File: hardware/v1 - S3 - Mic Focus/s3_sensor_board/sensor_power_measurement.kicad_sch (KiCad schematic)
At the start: 9 parts, among them J501 Conn_01x05, J502 Conn_01x05

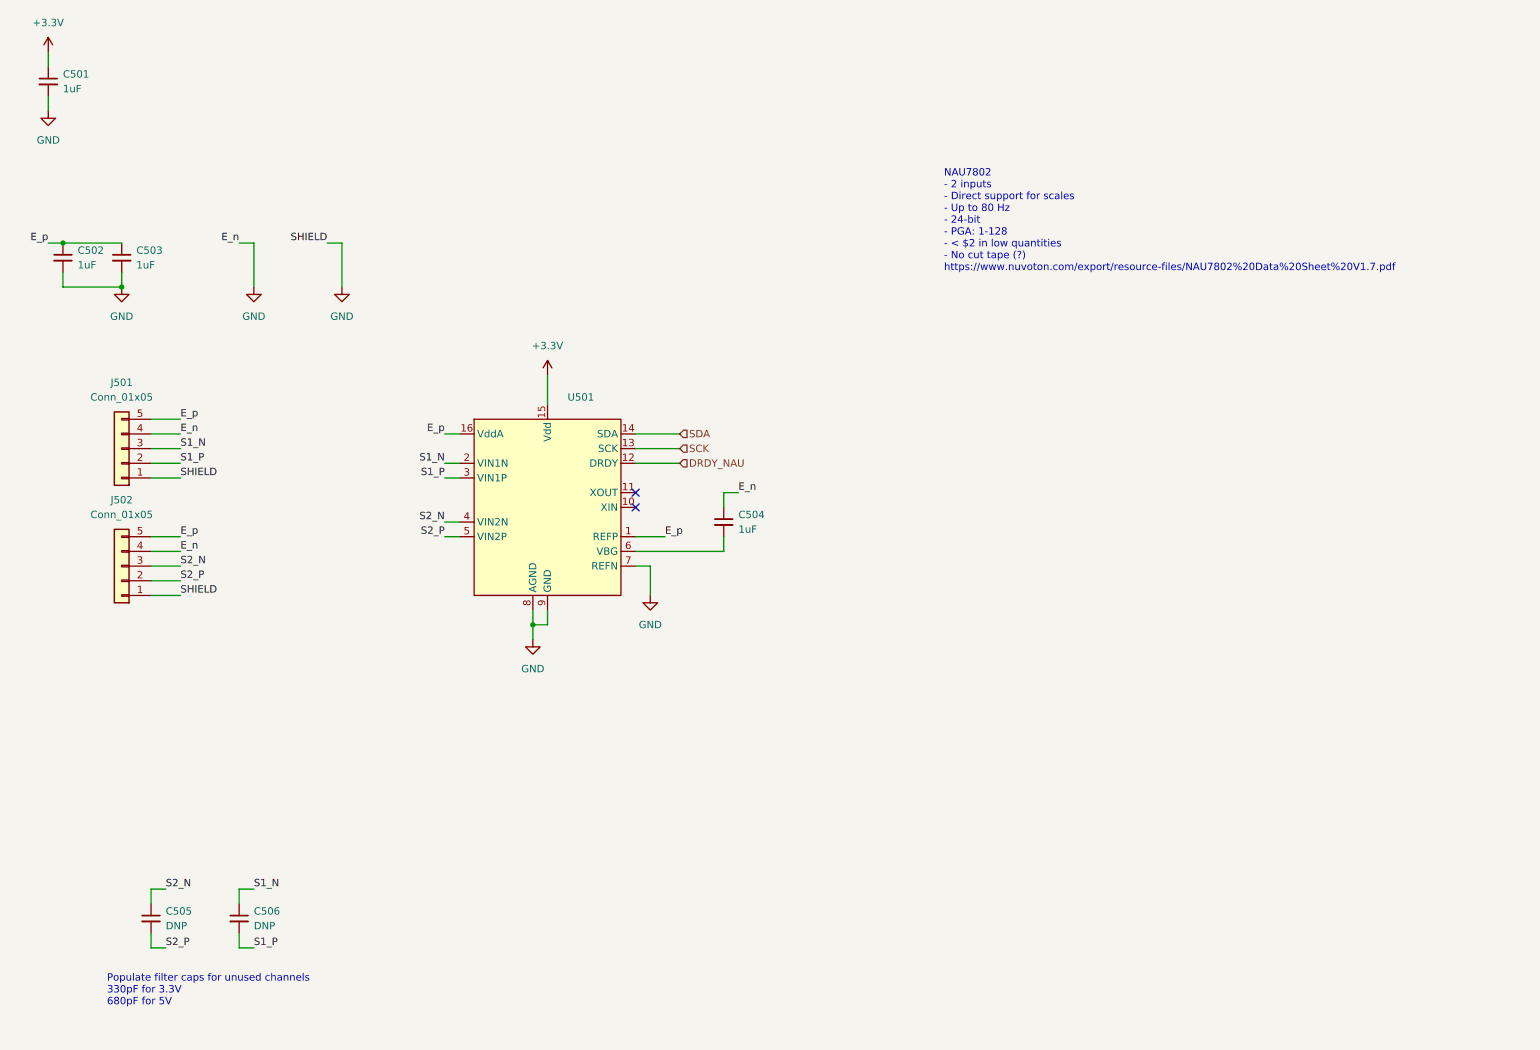
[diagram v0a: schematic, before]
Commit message: v1 board started
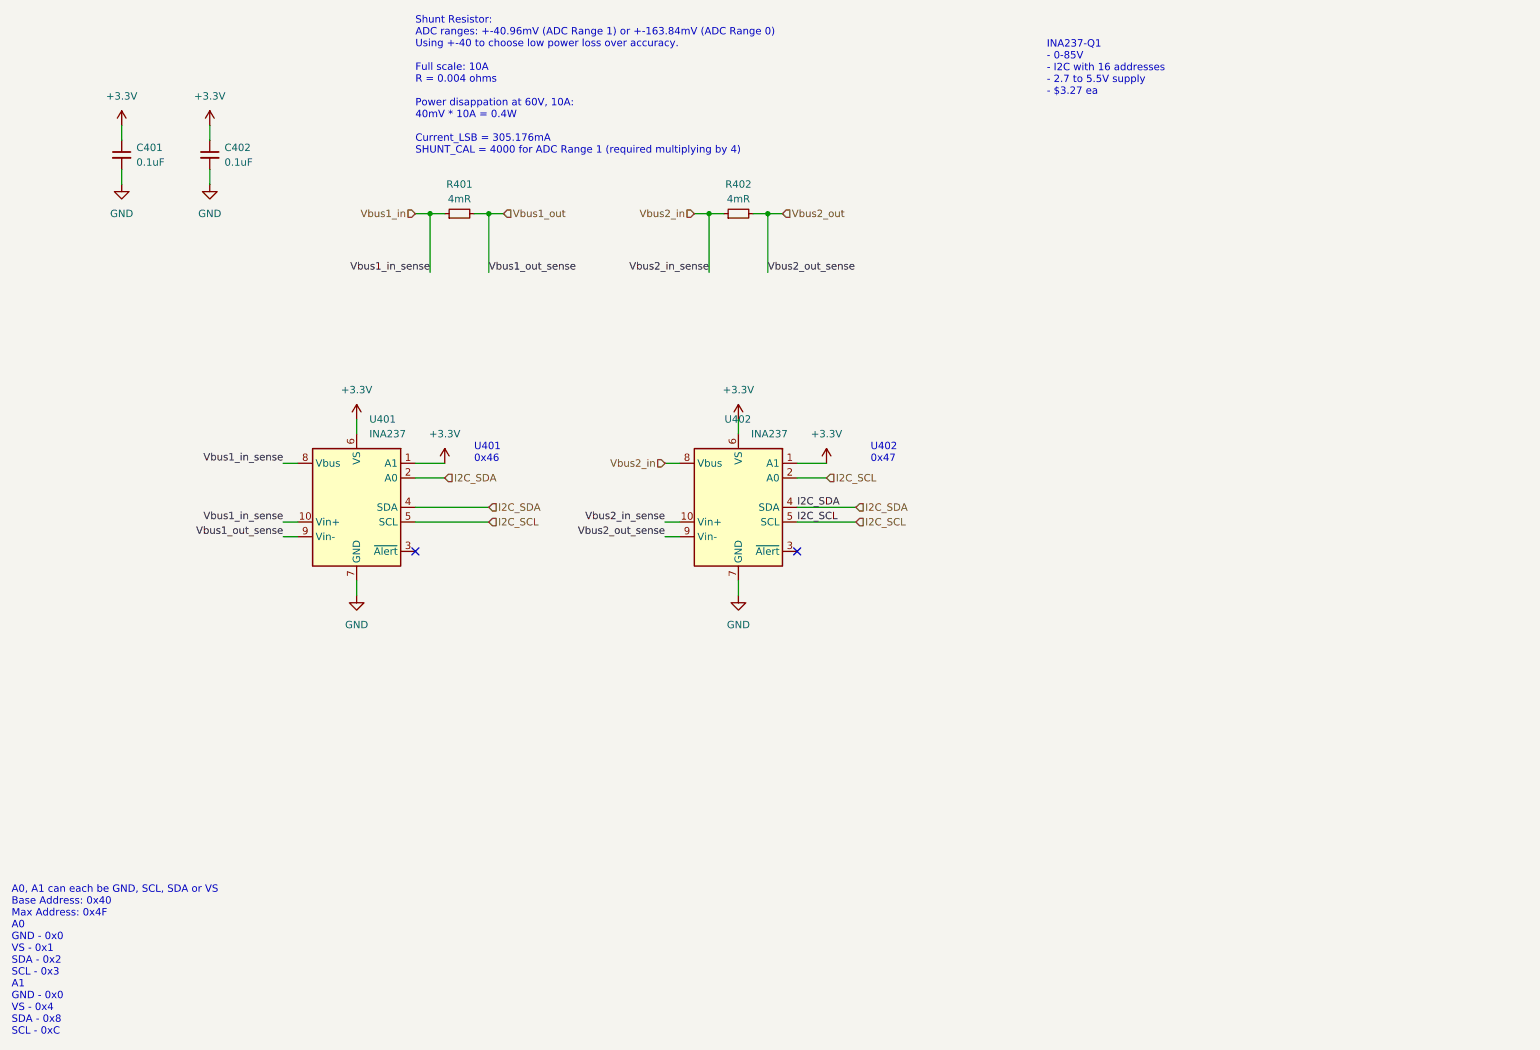
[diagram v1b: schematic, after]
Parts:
- removed C501, C502, C503, C504: 1uF, Capacitor_SMD:C_0805_2012Metric, symbol Device:C_Small
- removed C505, C506: DNP, Capacitor_SMD:C_0805_2012Metric, symbol Device:C_Small
- removed J501, J502: Conn_01x05, Connector_PinHeader_2.54mm:PinHeader_1x05_P2.54mm_Horizontal, symbol Connector_Generic:Conn_01x05
- removed U501: (no value), Package_SO:SOIC-16_3.9x9.9mm_P1.27mm, symbol BVH_Sensors:NAU7802
- added C401, C402: 0.1uF, Capacitor_SMD:C_0603_1608Metric, symbol Device:C_Small
- added R401, R402: 4mR, Resistor_SMD:R_2512_6332Metric, symbol Device:R_Small
- added U401, U402: INA237, Package_SO:VSSOP-10_3x3mm_P0.5mm, symbol BVH_Power:INA237
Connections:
- net +3.3V: now also C401.1, C402.1, U401.1 (A1), U401.6 (VS), U402.1 (A1), U402.6 (VS)
- net GND: now also C401.2, C402.2, U401.7 (GND), U402.7 (GND)
- new net I2C_SCL: U401.5 (SCL), U402.2 (A0), U402.5 (SCL)
- new net I2C_SDA: U401.2 (A0), U401.4 (SDA), U402.4 (SDA)
- new net Vbus1_in: R401.1, U401.10 (Vin+), U401.8 (Vbus)
- new net Vbus1_out: R401.2, U401.9 (Vin-)
- new net Vbus2_in: R402.1, U402.10 (Vin+), U402.8 (Vbus)
- new net Vbus2_out: R402.2, U402.9 (Vin-)
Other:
- note added: "A0, A1 can each be GND, SCL, SDA or VS Base Address: 0x40 Max Address: 0x4F A0 GND - 0x0 VS - 0x1 SDA - 0x2 SCL - 0x3 A1 GND - 0x0 VS - 0x4 SDA - 0x8 SCL - 0xC"
- note added: "INA237-Q1 - 0-85V - I2C with 16 addresses - 2.7 to 5.5V supply - $3.27 ea"
- note added: "Shunt Resistor: ADC ranges: +-40.96mV (ADC Range 1) or +-163.84mV (ADC Range 0) Using +-40 to choose low power loss over accuracy. Full scale: 10A R = 0.004 ohms Power disappation at 60V, 10A: 40mV * 10A = 0.4W Current_LSB = 305.176mA SHUNT_CAL = 4000 for ADC Range 1 (required multiplying by 4)"
- note added: "U401 0x46"
- note added: "U402 0x47"
- note removed: "NAU7802 - 2 inputs - Direct support for scales - Up to 80 Hz - 24-bit - PGA: 1-128 - < $2 in low quantities - No cut tape (?) https://www.nuvoton.com/export/resource-files/NAU7802%20Data%20Sheet%20V1.7.pdf"
- note removed: "Populate filter caps for unused channels 330pF for 3.3V 680pF for 5V"
